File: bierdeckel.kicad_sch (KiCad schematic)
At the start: 33 parts, among them SW1 Adress Coding, U1 TPS61201DRC, U2 ESP32-C3-WROOM-02

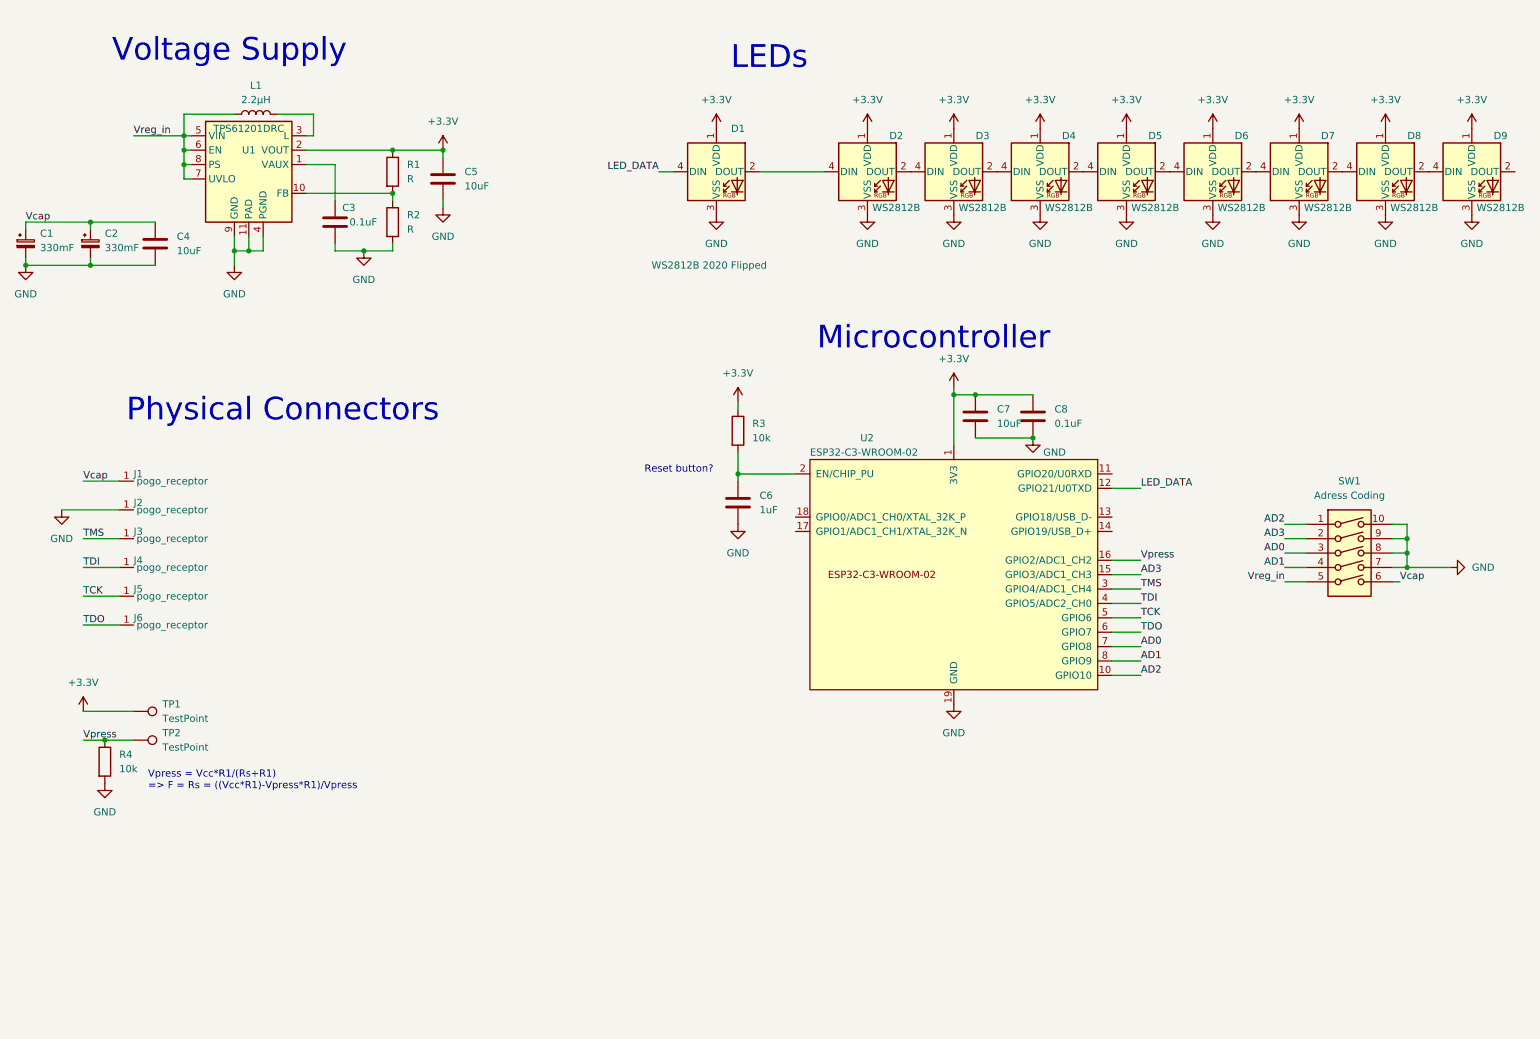
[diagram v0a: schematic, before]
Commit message: bla
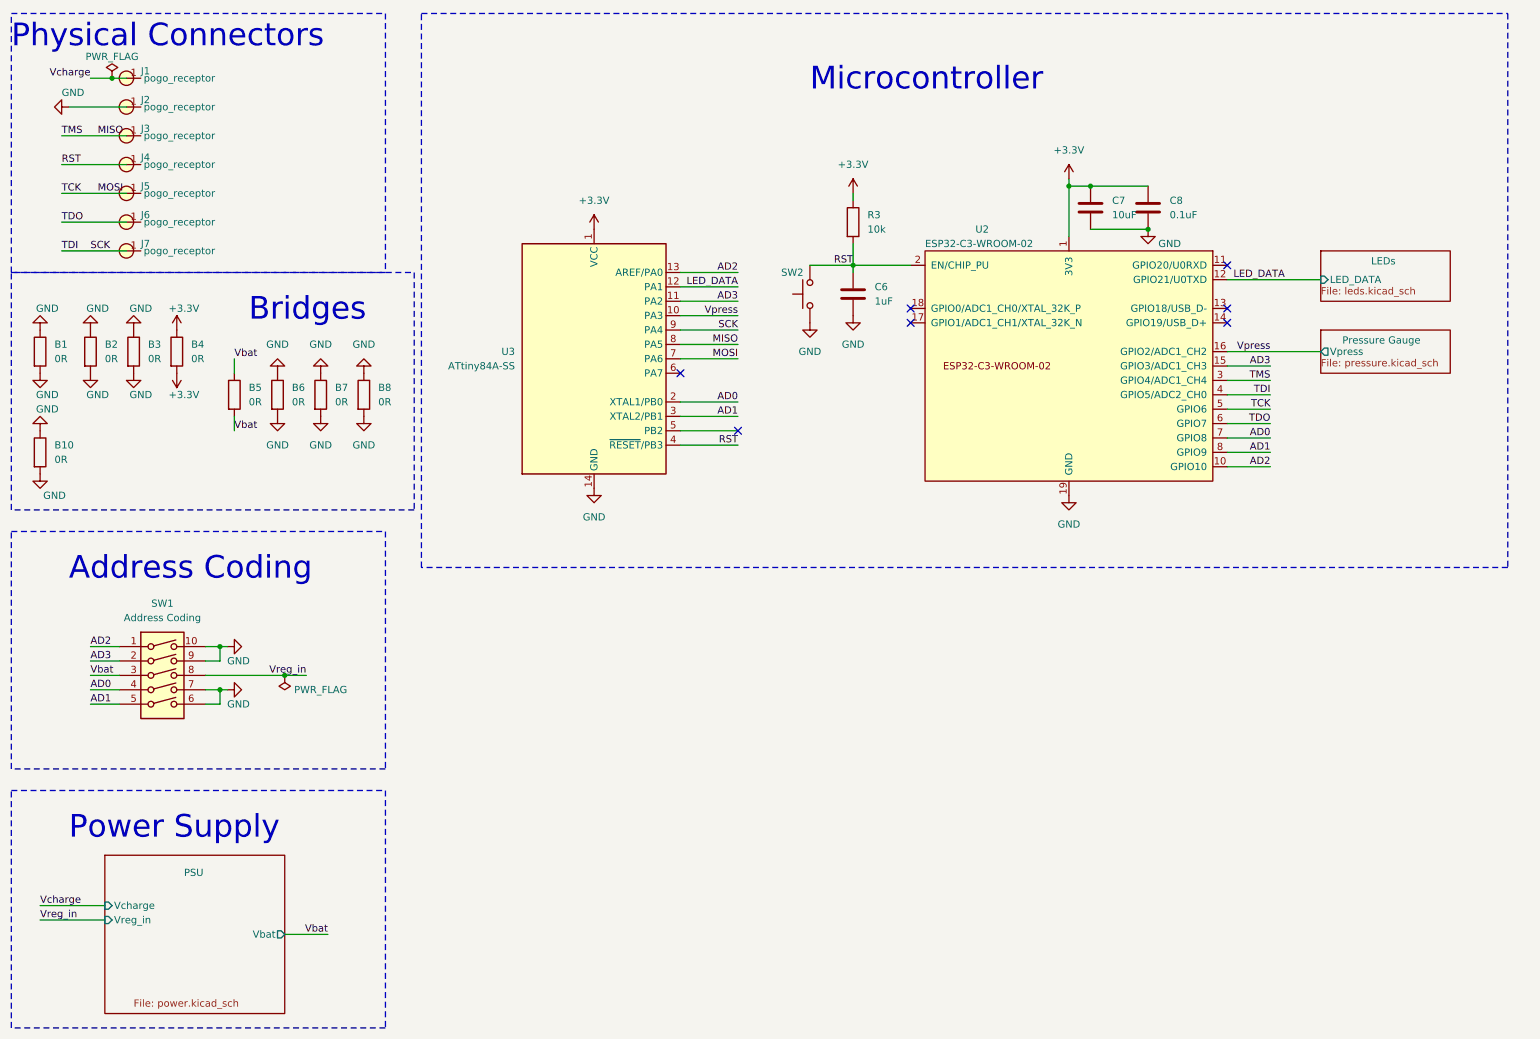
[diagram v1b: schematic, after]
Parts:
- removed C1, C2: 330mF, bier:super_cap, symbol bier:C_super
- removed C3: 0.1uF, Capacitor_SMD:C_0805_2012Metric, symbol Device:C
- removed C4, C5: 10uF, Capacitor_SMD:C_0805_2012Metric, symbol Device:C
- removed D1: WS2812B 2020 Flipped, bier:ws2812B_2020_flipped, symbol bier:WS2812B_2020_flipped
- removed D2, D3, D4, D5, D6, D7, D8, D9: WS2812B, LED_SMD:LED_WS2812B-2020_PLCC4_2.0x2.0mm, symbol LED:WS2812B
- removed L1: 2.2µH, Resistor_SMD:R_0805_2012Metric, symbol Device:L
- removed R1, R2: R, Resistor_SMD:R_0805_2012Metric, symbol Device:R
- removed R4: 10k, Resistor_SMD:R_0805_2012Metric, symbol Device:R
- removed TP1, TP2: TestPoint, TestPoint:TestPoint_Pad_D3.0mm, symbol Connector:TestPoint
- removed U1: TPS61201DRC, Package_SON:Texas_S-PVSON-N10_ThermalVias, symbol Regulator_Switching:TPS61201DRC
- added B1, B10, B2, B3, B4, B5, B6, B7, B8: 0R, Resistor_SMD:R_1206_3216Metric, symbol Device:R
- added J7: S70-332002045R, bier:pogo_receptor, symbol bier:Pogo_receptor
- added SW2: PTS526 SK15 SMTR2 LFS, Button_Switch_SMD:SW_Push_1P1T_XKB_TS-1187A, symbol Switch:SW_Push
- added U3: ATtiny84A-SS, Package_SO:SOIC-14_3.9x8.7mm_P1.27mm, symbol MCU_Microchip_ATtiny:ATtiny84A-SS
- C6: mpn (none) -> CL21B105KAFNNNG
- C7: mpn (none) -> CL21A106KPFNNNF
- C8: mpn (none) -> KGM21NR71H104KT
- J1, J2, J3, J4, J5, J6: value ~ -> S70-332002045R; mpn (none) -> S70-332002045R; now left out of the parts list
- R3: mpn (none) -> CR0805-FX-1002ELF
- SW1: value Adress Coding -> Address Coding; mpn (none) -> 219-5LPSTR
- U2: mpn (none) -> ESP32-C3-WROOM-02-N4
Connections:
- net +3.3V: now also B4.1, B4.2, U3.1 (VCC)
- net AD0: now also SW1.4, U3.2 (XTAL1/PB0); no longer SW1.3
- net AD1: now also SW1.5, U3.3 (XTAL2/PB1); no longer SW1.4
- net AD2: now also U3.13 (AREF/PA0)
- net AD3: now also U3.11 (PA2)
- net GND: now also SW1.6, B1.1, B1.2, B10.1, B10.2, B2.1, B2.2, B3.1, B3.2, B6.1, B6.2, B7.1, B7.2, B8.1, B8.2, SW2.1, U3.14 (GND); no longer SW1.8
- net LED_DATA: now also U3.12 (PA1)
- net Vpress: now also U3.10 (PA3)
- net Vreg_in: now also SW1.8; no longer SW1.5
- net RST: now reaches C6.1, R3.2, U2.2 (EN/CHIP_PU)
- net RST: now also J4.1 (pogo_receptor), SW2.2, U3.4 (~{RESET}/PB3)
- net TCK renamed MOSI
- net MOSI: now also U3.7 (PA6)
- net TDI renamed SCK
- net SCK: now also J7.1 (pogo_receptor), U3.9 (PA4); no longer J4.1 (pogo_receptor)
- net TMS renamed MISO
- net MISO: now also U3.8 (PA5)
- net Vcap renamed Vcharge
- net Vcharge: no longer SW1.6
- new net Vbat: B5.1, B5.2, SW1.3
- no-connect marks 0 -> 7
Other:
- added sheet LEDs (leds.kicad_sch)
- added sheet PSU (power.kicad_sch)
- added sheet Pressure Gauge (pressure.kicad_sch)
- note added: "Address Coding"
- note added: "Bridges"
- note added: "Power Supply"
- note removed: "LEDs"
- note removed: "Reset button?"
- note removed: "Voltage Supply"
- note removed: "Vpress = Vcc*R1/(Rs+R1) => F = Rs = ((Vcc*R1)-Vpress*R1)/Vpress"
- moved on the sheet: C6, C7, C8, R3, SW1, U2
